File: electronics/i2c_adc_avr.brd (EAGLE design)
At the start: 12.5 x 17.3 mm, 17 parts, among them IC1 TINY24/44/84-MU, IC2 TINY25/45/85-20MU

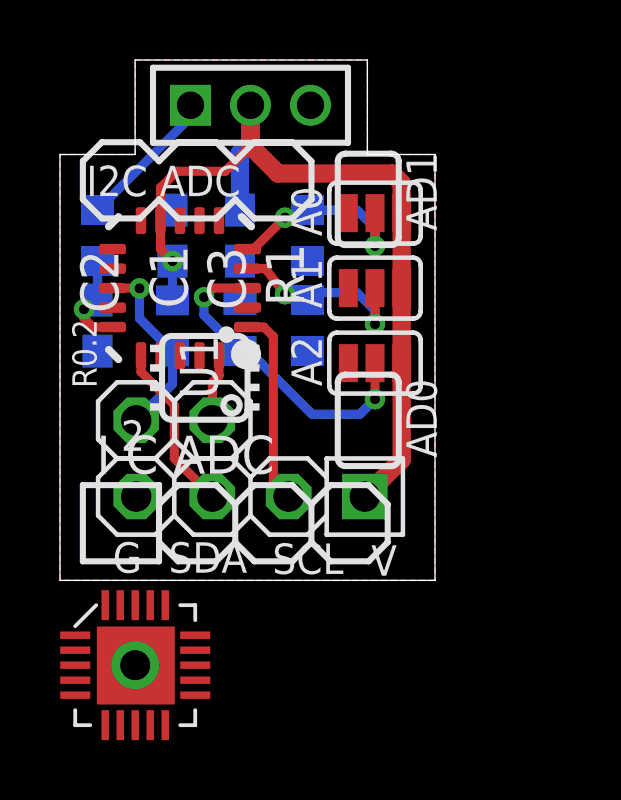
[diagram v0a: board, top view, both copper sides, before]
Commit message: Rev 0.3 as built (version is mislabeled on silk)
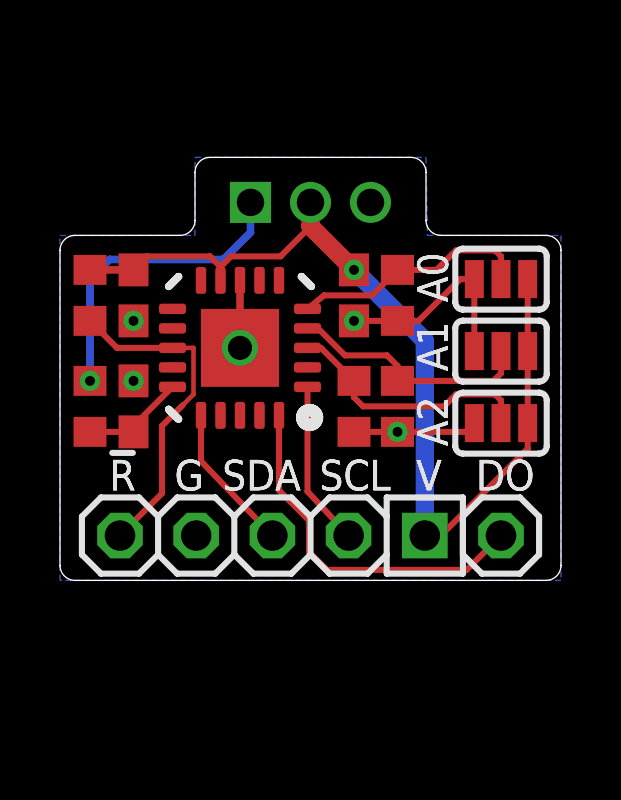
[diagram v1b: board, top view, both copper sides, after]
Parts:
- removed IC2: TINY25/45/85-20MU, mes_avr:20MLF
- C3: value 1uF -> 0.001uF
- JP5: value (none) -> MISO
- JP6: value (none) -> RESET
- JP7: value (none) -> MCU
- JP8: value (none) -> SIG
- R4: value 10 -> 10K
- moved JP5 10.4 mm to (14.7, 1.49)
- moved R4 5.70 mm to (1.00, 5.80), flipped to the top
- moved A0 4.74 mm to (14.7, 10.0)
- moved A1 4.70 mm to (14.7, 7.64)
- moved R2 4.66 mm to (9.80, 5.80), flipped to the top, turned to 90 degrees
- moved A2 4.65 mm to (14.7, 5.24)
- moved C4 4.29 mm to (9.80, 9.50), flipped to the top
- moved R1 4.03 mm to (11.2, 5.80), flipped to the top
- moved JP6 3.88 mm to (2.00, 1.49)
- moved JP8 3.81 mm to (8.35, 12.6), flipped to the bottom, turned to 180 degrees
- moved R0 3.60 mm to (11.2, 9.50), flipped to the top
- moved C3 2.95 mm to (2.45, 5.80), flipped to the top, turned to 90 degrees
- moved R3 2.93 mm to (1.00, 9.50), flipped to the top
- moved IC1 2.82 mm to (6.00, 7.75)
- moved JP7 2.39 mm to (8.35, 1.49)
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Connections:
- net !RESET: no longer IC2.1
- net A0: no longer IC2.12
- net A1: no longer IC2.2
- net AIN: no longer IC2.5
- net GND: now also IC1.GNDPAD; no longer IC2.8
- net SCL: no longer IC2.14
- net SDA: no longer IC2.11
- net VCC: no longer IC2.15
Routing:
- net GND: track 0.00 -> 13.4 mm, vias 0 -> 5
- net MISO: track 2.25 -> 12.1 mm
- net N$1: track 4.78 -> 10.4 mm, vias 0 -> 1
- net !RESET: track 6.44 -> 11.1 mm, vias 1 -> 0
- net VCC: track 29.0 -> 31.7 mm
- net A2: track 10.7 -> 8.59 mm, vias 2 -> 0
- net A1: track 6.73 -> 8.31 mm, vias 2 -> 0
- net A0: track 6.67 -> 8.07 mm, vias 2 -> 0
- net SCL: track 6.54 -> 5.50 mm
- net SDA: track 5.68 -> 4.96 mm
- net AIN: track 3.22 -> 3.49 mm, vias 1 -> 0
- removed copper zone on layer 1, net GND
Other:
- board size 12.5 x 17.3 mm -> 16.7 x 14.1 mm
- board text added: ""
- board text added: "A0"
- board text added: "A1"
- board text added: "A2"
- board text added: "http://ow.ly/m2JTf"
- board text removed: "2"
- board text removed: "AD0"
- board text removed: "AD1"
- board text removed: "C1"
- board text removed: "C2"
- board text removed: "C3"
- board text removed: "GND"
- board text removed: "I C ADC"
- board text removed: "I2C ADC"
- board text removed: "R1"
- board text removed: "SIG"
- board text removed: "U1"
- board text removed: "VCC"

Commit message: Changed footprint, layout
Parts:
- C3: value 0.001uF -> 1000pF
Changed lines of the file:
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@@
 <attribute name="NAME" x="12.93" y="6.971" size="1.016" layer="25" ratio="12" rot="R90"/>
 </element>
-<element name="C3" library="rcl" package="C0603" value="0.001uF" x="2.45" y="5.8" smashed="yes" rot="R90"/>
-<element name="C2" library="rcl" package="C0603" value="0.1uF" x="2.45" y="9.5" smashed="yes" rot="R270"/>
-<element name="R4" library="rcl" package="R0603" value="10K" x="1" y="5.8" smashed="yes" rot="R90"/>
+<element name="C3" library="rcl" package="C0603" value="1000pF" x="2.45" y="5.8" smashed="yes" rot="R90">
+<attribute name="PARTNO" value="CL10B102KB8SFNC" x="2.45" y="5.8" size="1.778" layer="27" rot="R90" display="off"/>
+<attribute name="CODE" value="102" x="2.45" y="5.8" size="1.778" layer="27" rot="R90" display="off"/>
+</element>
+<element name="C2" library="rcl" package="C0603" value="0.1uF" x="2.45" y="9.5" smashed="yes" rot="R270">
+<attribute name="PARTNO" value="C1608X7R1E104K080AA" x="2.45" y="9.5" size="1.778" layer="27" rot="R270" display="off"/>
+</element>
+<element name="R4" library="rcl" package="R0603" value="10K" x="1" y="5.8" smashed="yes" rot="R90">
+<attribute name="PARTNO" value="1622829-1" x="1" y="5.8" size="1.778" layer="27" rot="R90" display="off"/>
+</element>
 <element name="A0" library="SparkFun" package="SJ_3" value=" " x="14.7" y="10.042" smashed="yes">
 <attribute name="DATABASE" value="./../../eagle/PARTSDB.TXT" x="14.7" y="10.042" size="1.778" layer="27" display="off"/>
@@
 <attribute name="VALUE" x="13.43" y="8.137" size="0.4064" layer="27"/>
 </element>
-<element name="R0" library="rcl" package="R0603" value="220K" x="11.25" y="9.5" smashed="yes" rot="R90"/>
-<element name="R2" library="rcl" package="R0603" value="220K" x="9.8" y="5.8" smashed="yes" rot="R90"/>
+<element name="R0" library="rcl" package="R0603" value="220K" x="11.25" y="9.5" smashed="yes" rot="R90">
+<attribute name="PARTNO" value="RC1608J224CS" x="11.25" y="9.5" size="1.778" layer="27" rot="R90" display="off"/>
+</element>
+<element name="R2" library="rcl" package="R0603" value="220K" x="9.8" y="5.8" smashed="yes" rot="R90">
+<attribute name="PARTNO" value="RC1608J224CS" x="9.8" y="5.8" size="1.778" layer="27" rot="R90" display="off"/>
+</element>
 <element name="A2" library="SparkFun" package="SJ_3" value=" " x="14.7" y="5.242" smashed="yes">
 <attribute name="NAME" x="12.93" y="4.472" size="1.016" layer="25" ratio="12" rot="R90"/>
 </element>
-<element name="R1" library="rcl" package="R0603" value="220K" x="11.25" y="5.8" smashed="yes" rot="R90"/>
-<element name="C4" library="rcl" package="C0603" value="10uF" x="9.8" y="9.5" smashed="yes" rot="R270"/>
-<element name="IC1" library="avr-4" package="QFN/MLF20" value="TINY24/44/84-MU" x="6" y="7.75" smashed="yes" rot="R180"/>
-<element name="R3" library="rcl" package="R0603" value="10K" x="1" y="9.5" smashed="yes" rot="R90"/>
+<element name="R1" library="rcl" package="R0603" value="220K" x="11.25" y="5.8" smashed="yes" rot="R90">
+<attribute name="PARTNO" value="RC1608J224CS" x="11.25" y="5.8" size="1.778" layer="27" rot="R90" display="off"/>
+</element>
+<element name="C4" library="rcl" package="C0603" value="10uF" x="9.8" y="9.5" smashed="yes" rot="R270">
+<attribute name="PARTNO" value="CL10A106MP8NNNC" x="9.8" y="9.5" size="1.778" layer="27" rot="R270" display="off"/>
+</element>
+<element name="IC1" library="avr-4" package="QFN/MLF20" value="TINY24/44/84-MU" x="6" y="7.75" smashed="yes" rot="R180">
+<attribute name="PARTNO" value="ATTINY44A-MU" x="6" y="7.75" size="1.778" layer="27" rot="R180" display="off"/>
+</element>
+<element name="R3" library="rcl" package="R0603" value="10K" x="1" y="9.5" smashed="yes" rot="R90">
+<attribute name="PARTNO" value="1622829-1" x="1" y="9.5" size="1.778" layer="27" rot="R90" display="off"/>
+</element>
 <element name="JP5" library="pinhead-2" package="1X01" value="MISO" x="14.7" y="1.494" smashed="yes">
 <attribute name="VALUE" x="13.43" y="-1.681" size="1.27" layer="27"/>
